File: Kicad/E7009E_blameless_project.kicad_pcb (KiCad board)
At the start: 2 copper layers, 70.3 x 57.5 mm, 74 parts, among them M1 IRF9530, P1 CONN_01X06, P2 CONN_01X01, P3 CONN_01X01, P4 CONN_01X01, P5 CONN_01X01, Q1 BC556, Q10 BC546, Q11 BD135, Q12 BD136, Q13 IRF530, Q2 BC546, Q3 BC556, Q4 BC546, Q5 BC556, Q6 BC556, Q7 BC556, Q8 BC546, Q9 BD135

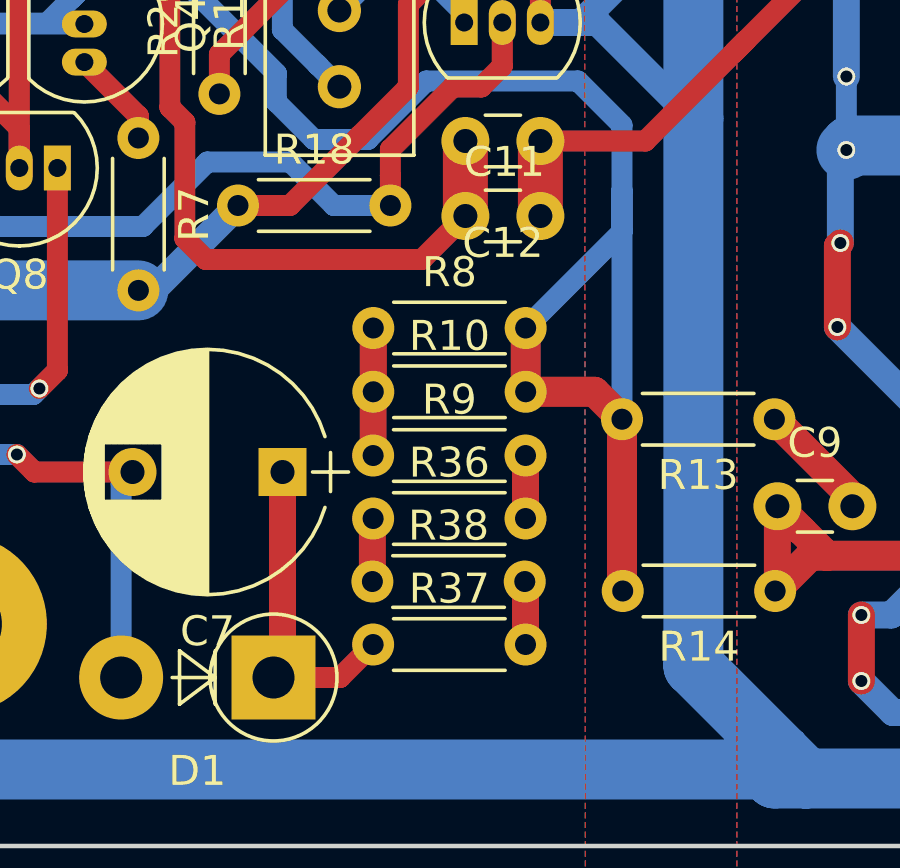
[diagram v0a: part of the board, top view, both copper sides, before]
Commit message: PNG's and stuff
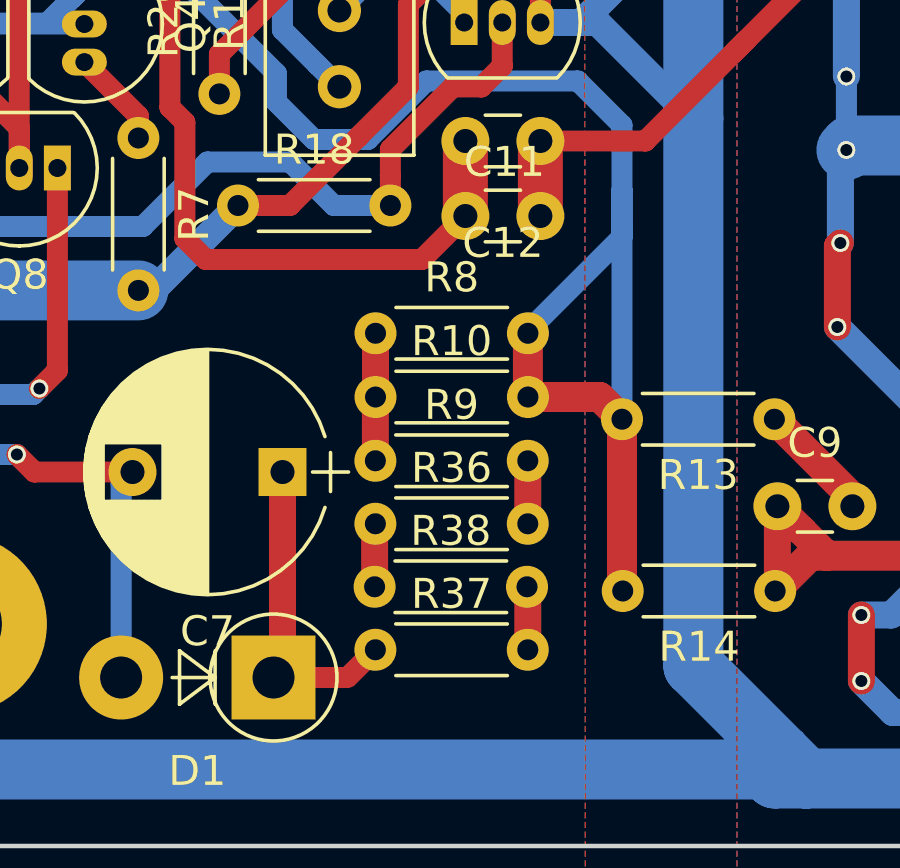
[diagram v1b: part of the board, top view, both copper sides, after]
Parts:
- moved R38 0.19 mm to (204.5, 117.6)
- moved R10 0.19 mm to (204.5, 111.3)
- moved R36 0.19 mm to (204.5, 115.5)
- moved R37 0.19 mm to (204.5, 119.7)
- moved R8 0.19 mm to (204.5, 109.2)
- moved R9 0.19 mm to (204.5, 113.4)
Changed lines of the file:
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@@
     (links 113)
     (no_connects 0)
-    (area 184.324555 68.674999 254.775001 126.325001)
+    (area 183.316667 55.134999 274.950983 127.000001)
     (thickness 1.6)
     (drawings 7)
-    (tracks 745)
+    (tracks 747)
     (zones 0)
     (modules 74)
@@
   )
   (setup
-    (last_trace_width 0.25)
+    (last_trace_width 1)
     (user_trace_width 0.3)
     (user_trace_width 0.4)
@@
   )
   (module Resistors_ThroughHole:R_Axial_DIN0204_L3.6mm_D1.6mm_P5.08mm_Horizontal (layer F.Cu)
-    (at 204.429653 108.984069)
+    (at 204.504653 109.159069)
     (descr "Resistor, Axial_DIN0204 series, Axial, Horizontal, pin pitch=5.08mm, 0.16666666666666666W = 1/6W, length*diameter=3.6*1.6mm^2, http://cdn-reichelt.de/documents/datenblatt/B400/1_4W%23YAG.pdf")
     (tags "Resistor Axial_DIN0204 series Axial Horizontal pin pitch 5.08mm 0.16666666666666666W = 1/6W length 3.6mm diameter 1.6mm")
@@
   )
   (module Resistors_ThroughHole:R_Axial_DIN0204_L3.6mm_D1.6mm_P5.08mm_Horizontal (layer F.Cu)
-    (at 204.424653 113.234069)
+    (at 204.499653 113.409069)
     (descr "Resistor, Axial_DIN0204 series, Axial, Horizontal, pin pitch=5.08mm, 0.16666666666666666W = 1/6W, length*diameter=3.6*1.6mm^2, http://cdn-reichelt.de/documents/datenblatt/B400/1_4W%23YAG.pdf")
     (tags "Resistor Axial_DIN0204 series Axial Horizontal pin pitch 5.08mm 0.16666666666666666W = 1/6W length 3.6mm diameter 1.6mm")
@@
   )
   (module Resistors_ThroughHole:R_Axial_DIN0204_L3.6mm_D1.6mm_P5.08mm_Horizontal (layer F.Cu)
-    (at 204.429653 111.109069)
+    (at 204.504653 111.284069)
     (descr "Resistor, Axial_DIN0204 series, Axial, Horizontal, pin pitch=5.08mm, 0.16666666666666666W = 1/6W, length*diameter=3.6*1.6mm^2, http://cdn-reichelt.de/documents/datenblatt/B400/1_4W%23YAG.pdf")
     (tags "Resistor Axial_DIN0204 series Axial Horizontal pin pitch 5.08mm 0.16666666666666666W = 1/6W length 3.6mm diameter 1.6mm")
@@
   )
   (module Resistors_ThroughHole:R_Axial_DIN0204_L3.6mm_D1.6mm_P5.08mm_Horizontal (layer F.Cu)
-    (at 204.424653 115.334069)
+    (at 204.499653 115.509069)
     (descr "Resistor, Axial_DIN0204 series, Axial, Horizontal, pin pitch=5.08mm, 0.16666666666666666W = 1/6W, length*diameter=3.6*1.6mm^2, http://cdn-reichelt.de/documents/datenblatt/B400/1_4W%23YAG.pdf")
     (tags "Resistor Axial_DIN0204 series Axial Horizontal pin pitch 5.08mm 0.16666666666666666W = 1/6W length 3.6mm diameter 1.6mm")
@@
   )
   (module Resistors_ThroughHole:R_Axial_DIN0204_L3.6mm_D1.6mm_P5.08mm_Horizontal (layer F.Cu)
-    (at 204.424653 119.534069)
+    (at 204.499653 119.709069)
     (descr "Resistor, Axial_DIN0204 series, Axial, Horizontal, pin pitch=5.08mm, 0.16666666666666666W = 1/6W, length*diameter=3.6*1.6mm^2, http://cdn-reichelt.de/documents/datenblatt/B400/1_4W%23YAG.pdf")
     (tags "Resistor Axial_DIN0204 series Axial Horizontal pin pitch 5.08mm 0.16666666666666666W = 1/6W length 3.6mm diameter 1.6mm")
@@
   )
   (module Resistors_ThroughHole:R_Axial_DIN0204_L3.6mm_D1.6mm_P5.08mm_Horizontal (layer F.Cu)
-    (at 204.399653 117.434069)
+    (at 204.474653 117.609069)
     (descr "Resistor, Axial_DIN0204 series, Axial, Horizontal, pin pitch=5.08mm, 0.16666666666666666W = 1/6W, length*diameter=3.6*1.6mm^2, http://cdn-reichelt.de/documents/datenblatt/B400/1_4W%23YAG.pdf")
     (tags "Resistor Axial_DIN0204 series Axial Horizontal pin pitch 5.08mm 0.16666666666666666W = 1/6W length 3.6mm diameter 1.6mm")
@@
   (segment (start 196.3 73.3) (end 196.3 70.85) (width 0.7) (layer F.Cu) (net 6))
   (segment (start 207.6 70.8) (end 206.05 70.8) (width 0.7) (layer F.Cu) (net 6))
-  (segment (start 201.104653 120.634069) (end 203.324653 120.634069) (width 0.7) (layer F.Cu) (net 7))
-  (segment (start 203.324653 120.634069) (end 204.424653 119.534069) (width 0.7) (layer F.Cu) (net 7))
+  (segment (start 201.104653 120.634069) (end 203.499653 120.634069) (width 0.7) (layer F.Cu) (net 7))
+  (segment (start 203.574653 120.634069) (end 204.499653 119.709069) (width 0.7) (layer F.Cu) (net 7))
   (segment (start 201.404653 113.784069) (end 201.404653 120.334069) (width 0.9) (layer F.Cu) (net 7))
   (segment (start 201.404653 120.334069) (end 201.104653 120.634069) (width 0.9) (layer F.Cu) (net 7))
@@
   (segment (start 196.6 102.65) (end 196.6 101.92) (width 0.7) (layer F.Cu) (net 27))
   (segment (start 196.6 101.92) (end 194.8 100.12) (width 0.7) (layer F.Cu) (net 27))
+  (segment (start 212.72 105.6) (end 212.72 112.025) (width 0.7) (layer B.Cu) (net 28))
+  (segment (start 212.72 104.4) (end 212.72 105.6) (width 0.7) (layer B.Cu) (net 28))
+  (segment (start 212.72 105.6) (end 212.72 105.948722) (width 0.7) (layer B.Cu) (net 28))
+  (segment (start 212.72 105.948722) (end 209.509653 109.159069) (width 0.7) (layer B.Cu) (net 28))
+  (segment (start 209.509653 111.284069) (end 211.979069 111.284069) (width 1) (layer F.Cu) (net 28))
+  (segment (start 211.979069 111.284069) (end 212.72 112.025) (width 1) (layer F.Cu) (net 28))
   (segment (start 212.72 102.22) (end 212.72 104.4) (width 0.7) (layer B.Cu) (net 28))
-  (segment (start 212.72 104.4) (end 212.72 112.025) (width 0.7) (layer B.Cu) (net 28))
-  (segment (start 209.509653 108.984069) (end 212.72 105.773722) (width 0.7) (layer B.Cu) (net 28))
   (segment (start 212.72 105.773722) (end 212.72 104.4) (width 0.7) (layer B.Cu) (net 28))
   (segment (start 195.5 93.18) (end 196.95 93.18) (width 0.7) (layer B.Cu) (net 28))
@@
   (segment (start 201.2 101.45) (end 202.45 102.7) (width 0.7) (layer B.Cu) (net 28))
   (segment (start 204.25 102.7) (end 206.2 100.75) (width 0.7) (layer B.Cu) (net 28))
-  (segment (start 209.509653 111.109069) (end 209.509653 108.984069) (width 1) (layer F.Cu) (net 28))
-  (segment (start 212.72 112.025) (end 211.804069 111.109069) (width 1) (layer F.Cu) (net 28))
-  (segment (start 211.804069 111.109069) (end 209.509653 111.109069) (width 1) (layer F.Cu) (net 28))
+  (segment (start 209.584653 111.284069) (end 209.584653 109.159069) (width 1) (layer F.Cu) (net 28))
   (segment (start 212.72 112.025) (end 212.72 117.725) (width 1) (layer F.Cu) (net 28))
   (segment (start 212.72 117.725) (end 212.745 117.75) (width 1) (layer F.Cu) (net 28))
@@
   (segment (start 252.672792 120.6) (end 251.4 120.6) (width 1.5) (layer B.Cu) (net 41))
   (segment (start 248.2 120.6) (end 251.4 120.6) (width 0.9) (layer F.Cu) (net 41))
-  (segment (start 204.429653 108.984069) (end 204.429653 111.109069) (width 0.9) (layer F.Cu) (net 42))
-  (segment (start 204.424653 113.234069) (end 204.424653 111.114069) (width 0.9) (layer F.Cu) (net 42))
-  (segment (start 204.424653 111.114069) (end 204.429653 111.109069) (width 0.9) (layer F.Cu) (net 42))
+  (segment (start 204.504653 109.159069) (end 204.504653 111.284069) (width 0.9) (layer F.Cu) (net 42))
+  (segment (start 204.499653 113.409069) (end 204.499653 111.289069) (width 0.9) (layer F.Cu) (net 42))
+  (segment (start 204.499653 111.289069) (end 204.504653 111.284069) (width 0.9) (layer F.Cu) (net 42))
   (segment (start 199.3 101.18) (end 199.3 99.86) (width 0.7) (layer F.Cu) (net 43))
   (segment (start 199.3 99.86) (end 203.3 95.86) (width 0.7) (layer F.Cu) (net 43))
-  (segment (start 209.504653 115.334069) (end 209.504653 113.234069) (width 0.9) (layer F.Cu) (net 44))
-  (segment (start 204.399653 117.434069) (end 204.399653 115.359069) (width 0.9) (layer F.Cu) (net 45))
-  (segment (start 204.399653 115.359069) (end 204.424653 115.334069) (width 0.9) (layer F.Cu) (net 45))
-  (segment (start 209.504653 119.534069) (end 209.504653 117.459069) (width 0.9) (layer F.Cu) (net 46))
-  (segment (start 209.504653 117.459069) (end 209.479653 117.434069) (width 0.9) (layer F.Cu) (net 46))
+  (segment (start 209.579653 115.509069) (end 209.579653 113.409069) (width 0.9) (layer F.Cu) (net 44))
+  (segment (start 204.474653 117.609069) (end 204.474653 115.534069) (width 0.9) (layer F.Cu) (net 45))
+  (segment (start 204.474653 115.534069) (end 204.499653 115.509069) (width 0.9) (layer F.Cu) (net 45))
+  (segment (start 209.579653 119.709069) (end 209.579653 117.634069) (width 0.9) (layer F.Cu) (net 46))
+  (segment (start 209.579653 117.634069) (end 209.554653 117.609069) (width 0.9) (layer F.Cu) (net 46))
   (zone (net 4) (net_name GNDPWR) (layer B.Cu) (hatch edge 0.508)
     (connect_pads (clearance 0.508))

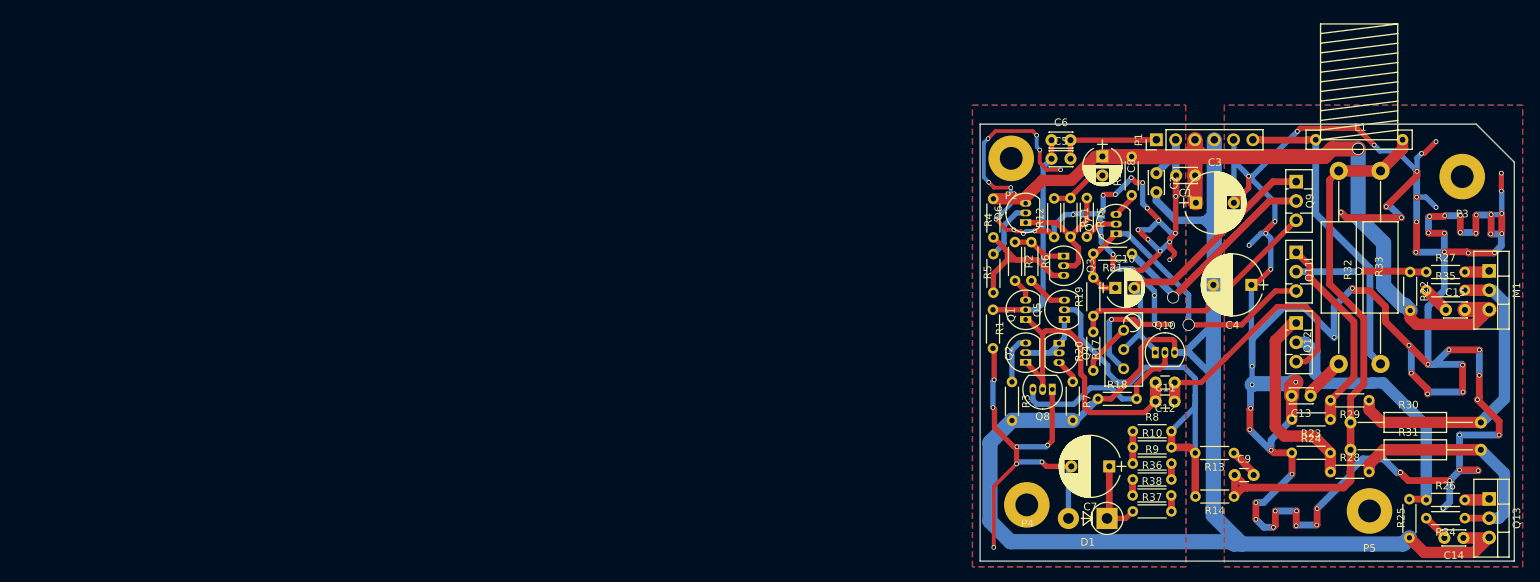
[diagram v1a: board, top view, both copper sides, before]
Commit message: All
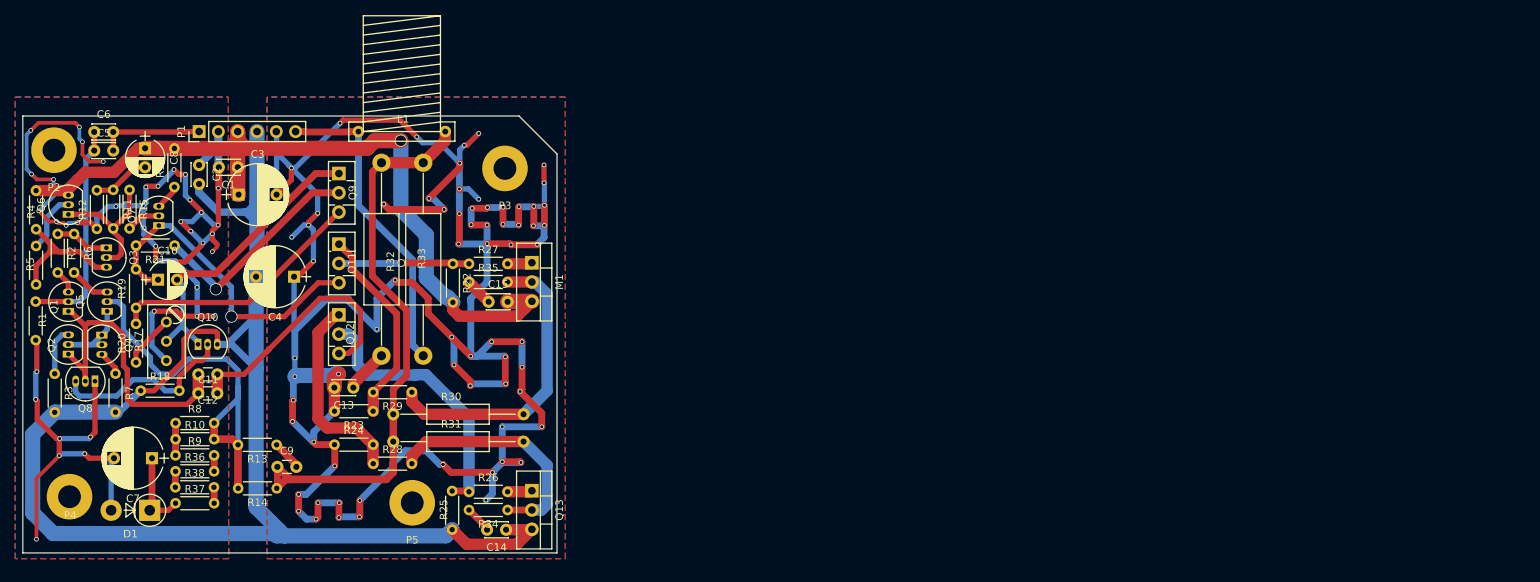
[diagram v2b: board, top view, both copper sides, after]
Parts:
- moved C13 126.0 mm to (101.9, 103.4)
- moved C3 126.0 mm to (86.8, 78.0)
- moved C5 126.0 mm to (67.8, 72.2)
- moved C6 126.0 mm to (67.8, 69.8)
- moved C9 126.0 mm to (91.9, 113.8)
- moved D1 126.0 mm to (75.1, 119.6)
- moved M1 126.0 mm to (125.4, 87.0)
- moved P4 126.0 mm to (64.6, 117.8)
- moved P5 126.0 mm to (109.7, 118.6)
- moved Q1 126.0 mm to (64.4, 93.4)
- moved Q10 126.0 mm to (81.5, 97.7)
- moved Q13 126.0 mm to (125.4, 117.0)
- moved Q2 126.0 mm to (64.4, 99.0)
- moved Q3 126.0 mm to (69.4, 85.0)
- moved Q4 126.0 mm to (68.8, 96.5)
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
